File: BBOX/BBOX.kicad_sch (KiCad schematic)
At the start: 20 parts, among them J1 BBOX, J10 LED, J2 WJ127-5.0-2P, J3 Servo2, J7 IR_LEDs, J9 Servo1, Q1 IRLML2502PBF, U2 AP2210N-3.3TRG1, U4 PCA9685PW, U5 PCA9306

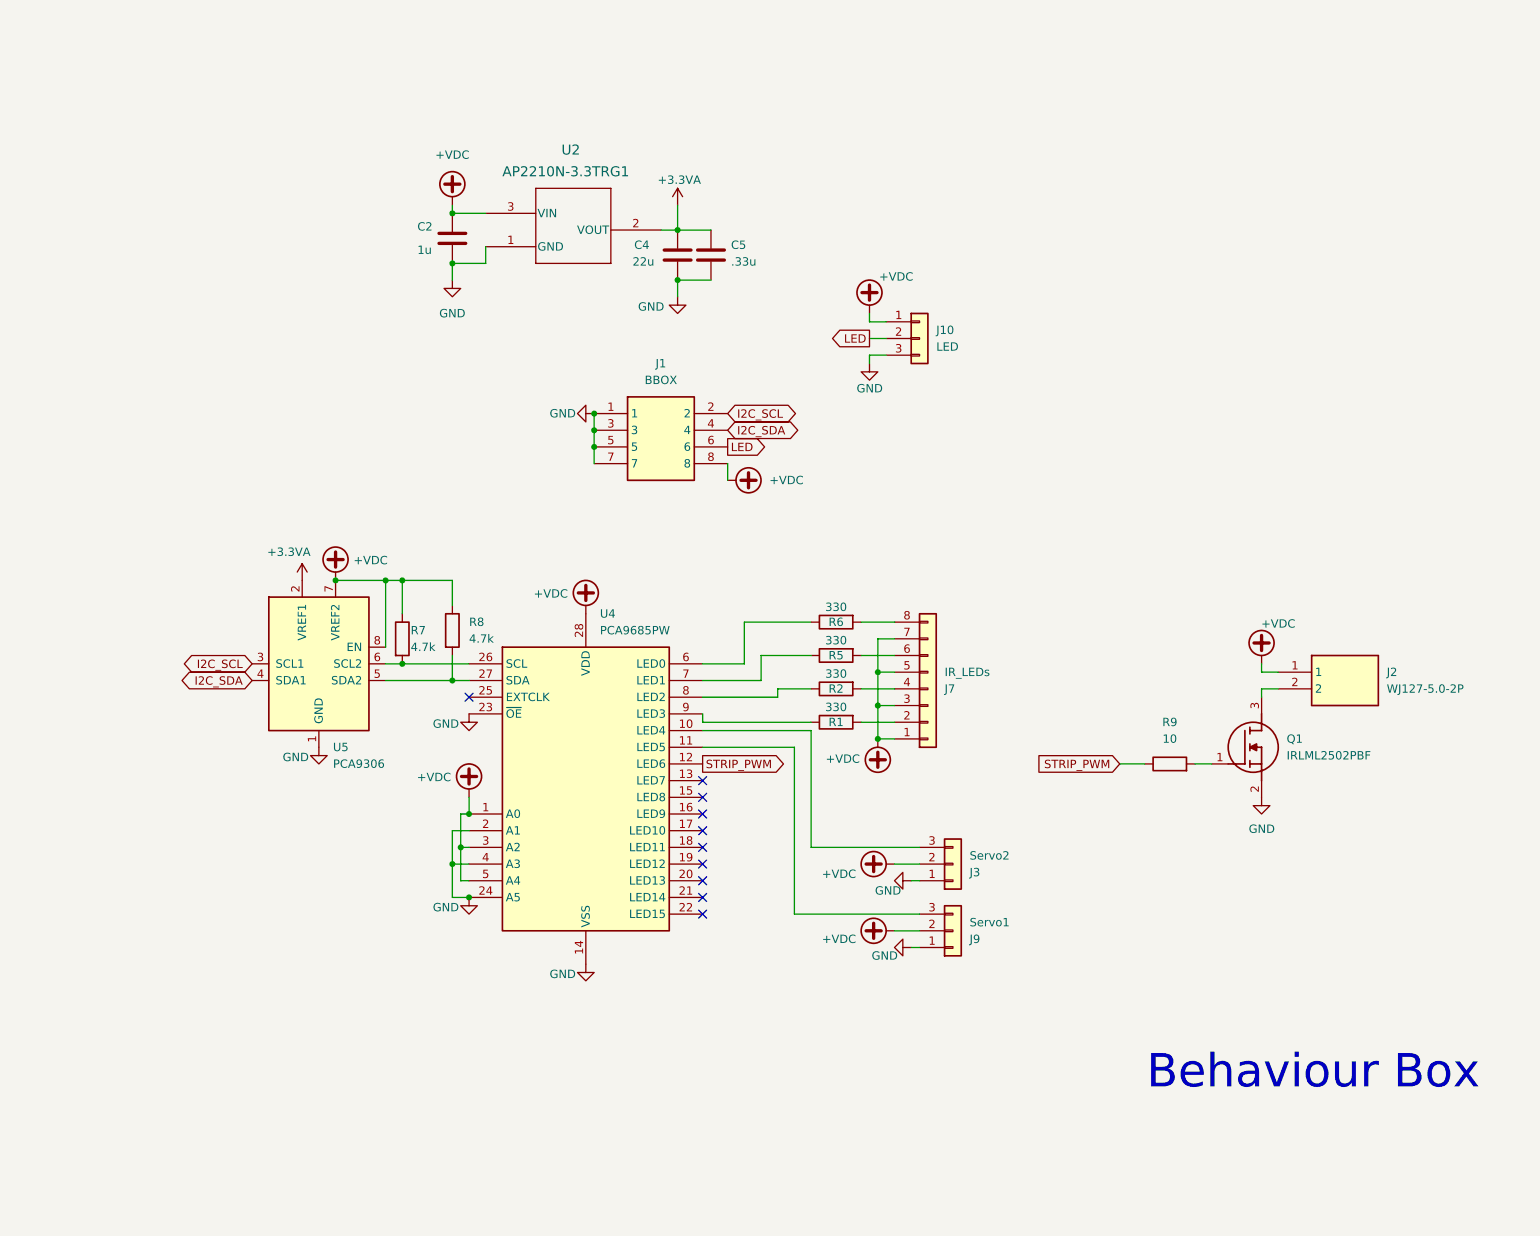
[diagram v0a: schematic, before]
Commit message: v1.0
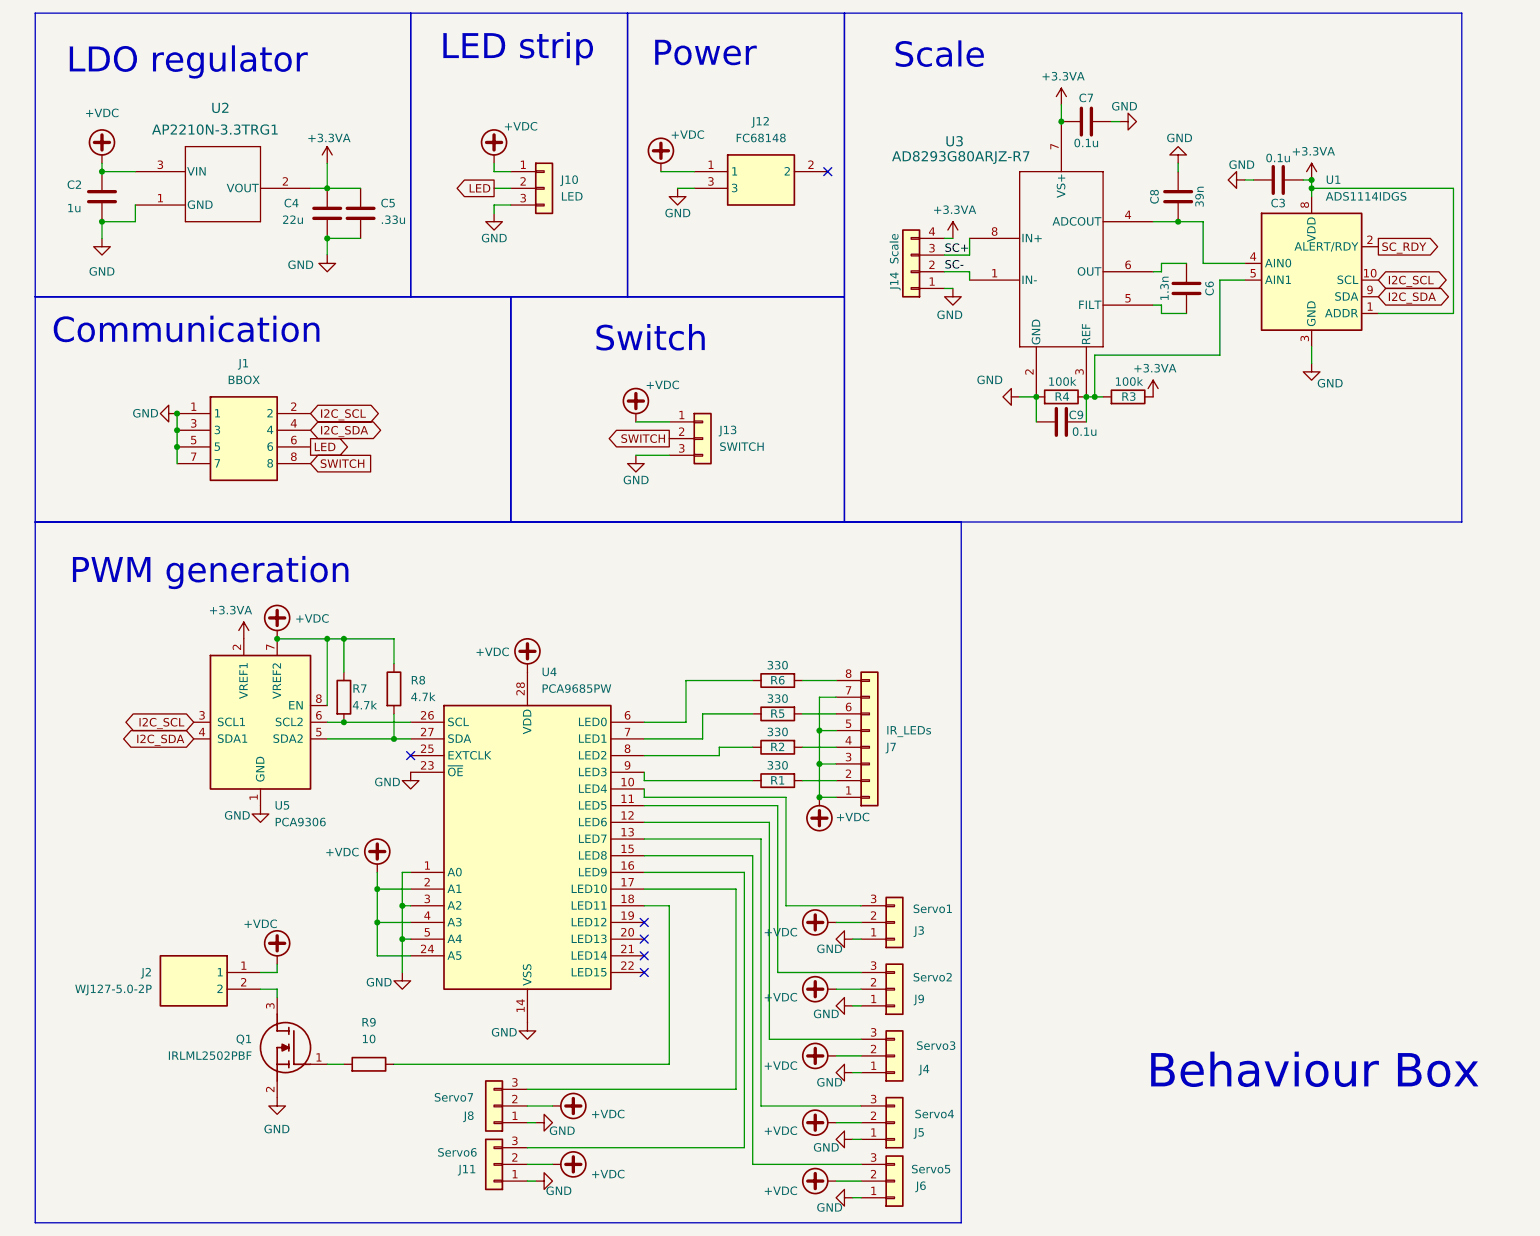
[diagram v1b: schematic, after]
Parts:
- added C3, C7, C9: 0.1u, Capacitor_SMD:C_1206_3216Metric_Pad1.33x1.80mm_HandSolder, symbol Device:C
- added C6: 1.3n, Capacitor_SMD:C_1206_3216Metric_Pad1.33x1.80mm_HandSolder, symbol Device:C
- added C8: 39n, Capacitor_SMD:C_1206_3216Metric_Pad1.33x1.80mm_HandSolder, symbol Device:C
- added J11: Servo6, Connector_PinHeader_2.54mm:PinHeader_1x03_P2.54mm_Vertical, symbol Connector_Generic:Conn_01x03
- added J12: FC68148, FC68148:FC68148, symbol FC68148:FC68148
- added J13: SWITCH, Connector_PinHeader_2.54mm:PinHeader_1x03_P2.54mm_Vertical, symbol Connector_Generic:Conn_01x03
- added J14: Scale, JL308-25404G01:JL308-25404G01, symbol Connector_Generic:Conn_01x04
- added J4: Servo3, Connector_PinHeader_2.54mm:PinHeader_1x03_P2.54mm_Vertical, symbol Connector_Generic:Conn_01x03
- added J5: Servo4, Connector_PinHeader_2.54mm:PinHeader_1x03_P2.54mm_Vertical, symbol Connector_Generic:Conn_01x03
- added J6: Servo5, Connector_PinHeader_2.54mm:PinHeader_1x03_P2.54mm_Vertical, symbol Connector_Generic:Conn_01x03
- added J8: Servo7, Connector_PinHeader_2.54mm:PinHeader_1x03_P2.54mm_Vertical, symbol Connector_Generic:Conn_01x03
- added R3, R4: 100k, Resistor_SMD:R_1206_3216Metric_Pad1.30x1.75mm_HandSolder, symbol Device:R
- added U1: ADS1114IDGS, ADS1114IDGST:DGS10, symbol Analog_ADC:ADS1114IDGS
- added U3: AD8293G80ARJZ-R7, AD8293G80ARJZ-R7:RJ_8_ADI, symbol AD8293G80ARJZ-R7:AD8293G80ARJZ-R7
- J3: value Servo2 -> Servo1
- J9: value Servo1 -> Servo2
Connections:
- net +3.3VA: now also C3.2, C7.2, J14.4 (Pin_4), R3.1, U1.1 (ADDR), U1.8 (VDD), U3.7 (VS+)
- net +VDC: now also U4.2 (A1), U4.24 (A5), U4.4 (A3), J11.2 (Pin_2), J12.1, J13.1 (Pin_1), J4.2 (Pin_2), J5.2 (Pin_2), J6.2 (Pin_2), J8.2 (Pin_2); no longer J1.8, U4.1 (A0), U4.3 (A2), U4.5 (A4)
- net GND: now also U4.1 (A0), U4.3 (A2), U4.5 (A4), C3.1, C7.1, C8.1, C9.2, J11.1 (Pin_1), J12.3, J13.3 (Pin_3), J14.1 (Pin_1), J4.1 (Pin_1), J5.1 (Pin_1), J6.1 (Pin_1), J8.1 (Pin_1), R4.2, U1.3 (GND), U3.2 (GND); no longer U4.2 (A1), U4.24 (A5), U4.4 (A3)
- net I2C_SCL: now also U1.10 (SCL)
- net I2C_SDA: now also U1.9 (SDA)
- net at U4.13 (LED7): now also J5.3 (Pin_3)
- net at U4.15 (LED8): now also J6.3 (Pin_3)
- net at U4.16 (LED9): now also J11.3 (Pin_3)
- net at U4.17 (LED10): now also J8.3 (Pin_3)
- net at U4.18 (LED11): now also R9.1
- net STRIP_PWM: no longer names the net of U4.12 (LED6)
- net STRIP_PWM: now also J4.3 (Pin_3); no longer R9.1
- new net: C9.1, R3.2, R4.1, U1.5 (AIN1), U3.3 (REF)
- new net: C8.2, U1.4 (AIN0), U3.4 (ADCOUT)
- new net: C6.1, U3.5 (FILT)
- new net: C6.2, U3.6 (OUT)
- new net SC+: J14.3 (Pin_3), U3.8 (IN+)
- new net SC-: J14.2 (Pin_2), U3.1 (IN-)
- new net SC_RDY: U1.2 (ALERT/RDY)
- new net SWITCH: J1.8, J13.2 (Pin_2)
- no-connect marks 10 -> 6
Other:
- note added: "Communication"
- note added: "LDO regulator"
- note added: "LED strip"
- note added: "PWM generation"
- note added: "Power"
- note added: "Scale"
- note added: "Switch"
- moved on the sheet: C2, C4, C5, J1, J10, J2, J3, J7, J9, Q1, R1, R2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
